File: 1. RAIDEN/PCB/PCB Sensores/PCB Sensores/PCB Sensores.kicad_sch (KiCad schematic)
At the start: 19 parts, among them J2 LEDS_1, J3 LEDS_1, J4 LEDS_1, U1 BOB-09056

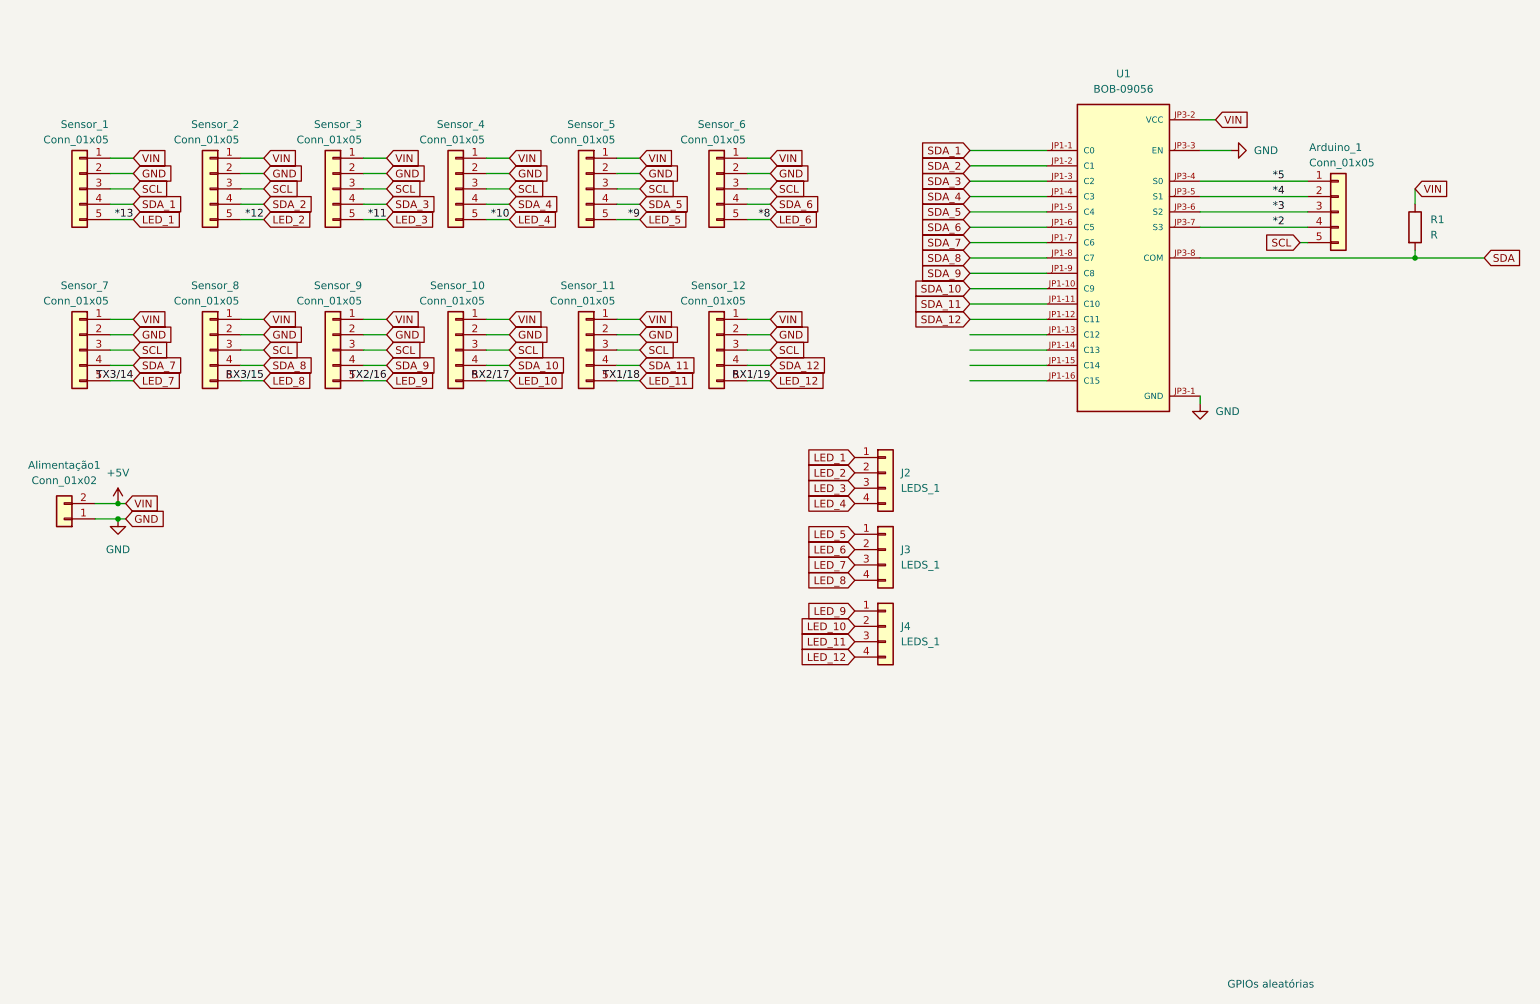
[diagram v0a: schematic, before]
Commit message: V2 da PCB dos sensores
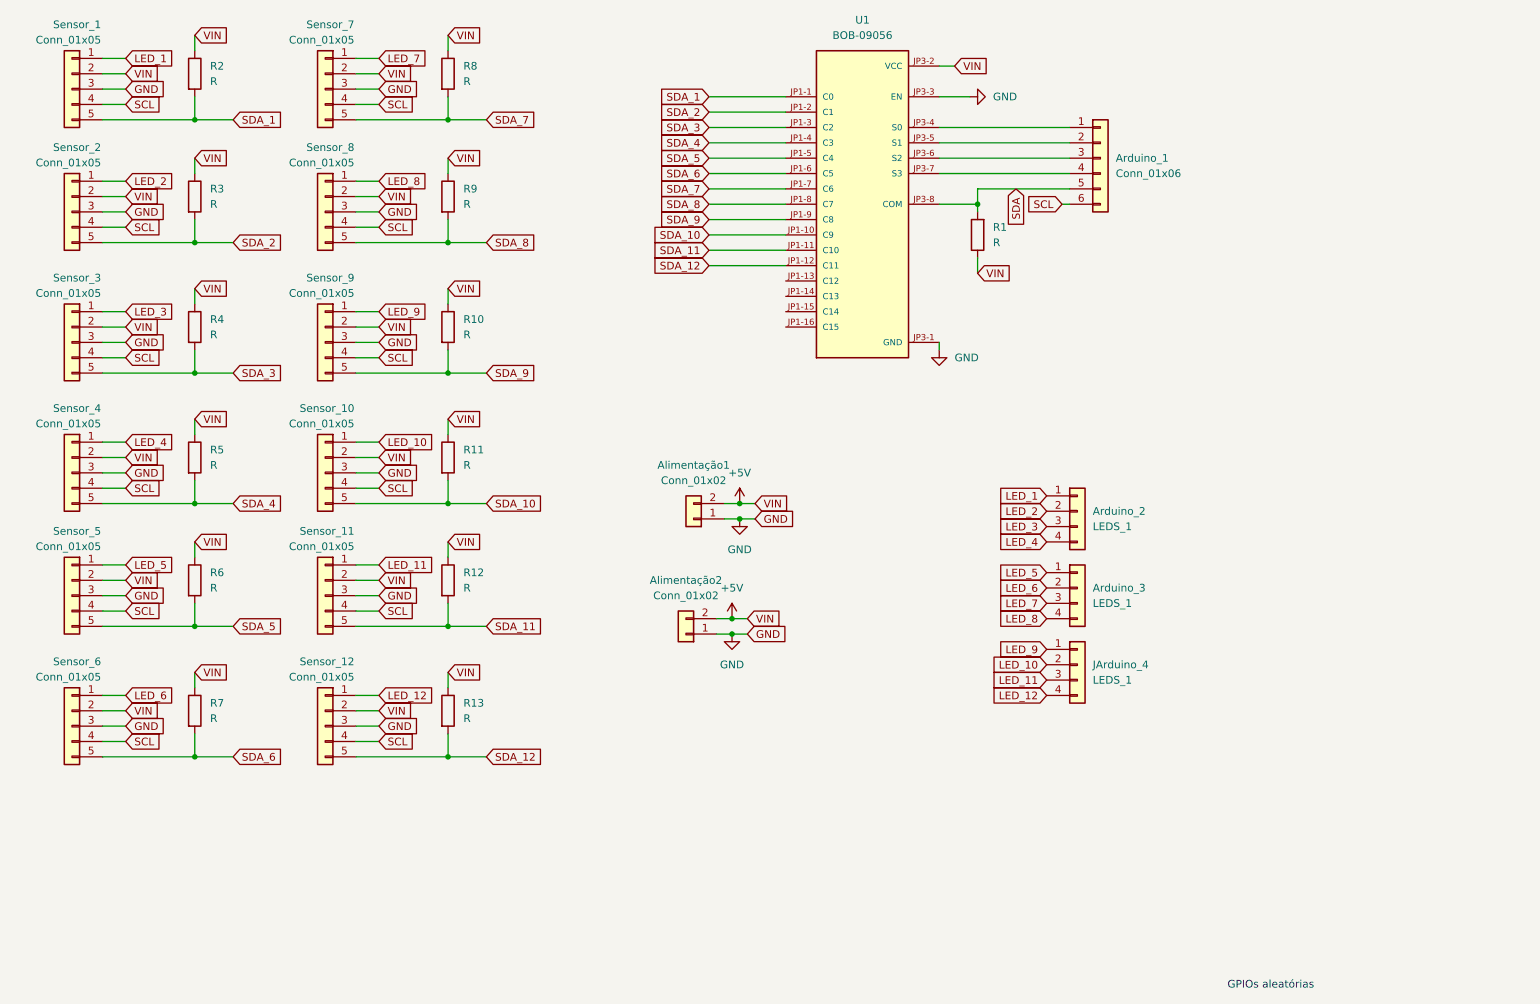
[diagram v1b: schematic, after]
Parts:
- removed Arduino_1: Conn_01x05, Connector_PinSocket_2.54mm:PinSocket_1x05_P2.54mm_Vertical, symbol Connector_Generic:Conn_01x05
- added Alimentação2: Conn_01x02, Connector_PinSocket_2.54mm:PinSocket_1x02_P2.54mm_Vertical, symbol Connector_Generic:Conn_01x02
- added Arduino_1: Conn_01x06, Connector_PinHeader_2.54mm:PinHeader_1x06_P2.54mm_Vertical, symbol Connector_Generic:Conn_01x06
- added R10, R11, R12, R13, R2, R3, R4, R5, R6, R7, R8, R9: R, Resistor_THT:R_Axial_DIN0207_L6.3mm_D2.5mm_P7.62mm_Horizontal, symbol Device:R
- renumbered J2 to Arduino_2, J3 to Arduino_3, J4 to JArduino_4
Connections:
- net +5V: now also Sensor_1.2 (Pin_2), Sensor_10.2 (Pin_2), Sensor_11.2 (Pin_2), Sensor_12.2 (Pin_2), Sensor_2.2 (Pin_2), Sensor_3.2 (Pin_2), Sensor_4.2 (Pin_2), Sensor_5.2 (Pin_2), Sensor_6.2 (Pin_2), Sensor_7.2 (Pin_2), Sensor_8.2 (Pin_2), Sensor_9.2 (Pin_2), Alimentação2.2 (Pin_2), R10.1, R11.1, R12.1, R13.1, R2.1, R3.1, R4.1, R5.1, R6.1, R7.1, R8.1, R9.1; no longer Sensor_1.1 (Pin_1), Sensor_10.1 (Pin_1), Sensor_11.1 (Pin_1), Sensor_12.1 (Pin_1), Sensor_2.1 (Pin_1), Sensor_3.1 (Pin_1), Sensor_4.1 (Pin_1), Sensor_5.1 (Pin_1), Sensor_6.1 (Pin_1), Sensor_7.1 (Pin_1), Sensor_8.1 (Pin_1), Sensor_9.1 (Pin_1)
- net GND: now also Sensor_1.3 (Pin_3), Sensor_10.3 (Pin_3), Sensor_11.3 (Pin_3), Sensor_12.3 (Pin_3), Sensor_2.3 (Pin_3), Sensor_3.3 (Pin_3), Sensor_4.3 (Pin_3), Sensor_5.3 (Pin_3), Sensor_6.3 (Pin_3), Sensor_7.3 (Pin_3), Sensor_8.3 (Pin_3), Sensor_9.3 (Pin_3), Alimentação2.1 (Pin_1); no longer Sensor_1.2 (Pin_2), Sensor_10.2 (Pin_2), Sensor_11.2 (Pin_2), Sensor_12.2 (Pin_2), Sensor_2.2 (Pin_2), Sensor_3.2 (Pin_2), Sensor_4.2 (Pin_2), Sensor_5.2 (Pin_2), Sensor_6.2 (Pin_2), Sensor_7.2 (Pin_2), Sensor_8.2 (Pin_2), Sensor_9.2 (Pin_2)
- net LED_1: now also Sensor_1.1 (Pin_1); no longer Sensor_1.5 (Pin_5)
- net LED_10: now also Sensor_10.1 (Pin_1); no longer Sensor_10.5 (Pin_5)
- net LED_11: now also Sensor_11.1 (Pin_1); no longer Sensor_11.5 (Pin_5)
- net LED_12: now also Sensor_12.1 (Pin_1); no longer Sensor_12.5 (Pin_5)
- net LED_2: now also Sensor_2.1 (Pin_1); no longer Sensor_2.5 (Pin_5)
- net LED_3: now also Sensor_3.1 (Pin_1); no longer Sensor_3.5 (Pin_5)
- net LED_4: now also Sensor_4.1 (Pin_1); no longer Sensor_4.5 (Pin_5)
- net LED_5: now also Sensor_5.1 (Pin_1); no longer Sensor_5.5 (Pin_5)
- net LED_6: now also Sensor_6.1 (Pin_1); no longer Sensor_6.5 (Pin_5)
- net LED_7: now also Sensor_7.1 (Pin_1); no longer Sensor_7.5 (Pin_5)
- net LED_8: now also Sensor_8.1 (Pin_1); no longer Sensor_8.5 (Pin_5)
- net LED_9: now also Sensor_9.1 (Pin_1); no longer Sensor_9.5 (Pin_5)
- net SCL: now also Sensor_1.4 (Pin_4), Sensor_10.4 (Pin_4), Sensor_11.4 (Pin_4), Sensor_12.4 (Pin_4), Sensor_2.4 (Pin_4), Sensor_3.4 (Pin_4), Sensor_4.4 (Pin_4), Sensor_5.4 (Pin_4), Sensor_6.4 (Pin_4), Sensor_7.4 (Pin_4), Sensor_8.4 (Pin_4), Sensor_9.4 (Pin_4), Arduino_1.6 (Pin_6); no longer Sensor_1.3 (Pin_3), Sensor_10.3 (Pin_3), Sensor_11.3 (Pin_3), Sensor_12.3 (Pin_3), Sensor_2.3 (Pin_3), Sensor_3.3 (Pin_3), Sensor_4.3 (Pin_3), Sensor_5.3 (Pin_3), Sensor_6.3 (Pin_3), Sensor_7.3 (Pin_3), Sensor_8.3 (Pin_3), Sensor_9.3 (Pin_3)
- net SDA: now also Arduino_1.5 (Pin_5)
- net SDA_1: now also Sensor_1.5 (Pin_5), R2.2; no longer Sensor_1.4 (Pin_4)
- net SDA_10: now also Sensor_10.5 (Pin_5), R11.2; no longer Sensor_10.4 (Pin_4)
- net SDA_11: now also Sensor_11.5 (Pin_5), R12.2; no longer Sensor_11.4 (Pin_4)
- net SDA_12: now also Sensor_12.5 (Pin_5), R13.2; no longer Sensor_12.4 (Pin_4)
- net SDA_2: now also Sensor_2.5 (Pin_5), R3.2; no longer Sensor_2.4 (Pin_4)
- net SDA_3: now also Sensor_3.5 (Pin_5), R4.2; no longer Sensor_3.4 (Pin_4)
- net SDA_4: now also Sensor_4.5 (Pin_5), R5.2; no longer Sensor_4.4 (Pin_4)
- net SDA_5: now also Sensor_5.5 (Pin_5), R6.2; no longer Sensor_5.4 (Pin_4)
- net SDA_6: now also Sensor_6.5 (Pin_5), R7.2; no longer Sensor_6.4 (Pin_4)
- net SDA_7: now also Sensor_7.5 (Pin_5), R8.2; no longer Sensor_7.4 (Pin_4)
- net SDA_8: now also Sensor_8.5 (Pin_5), R9.2; no longer Sensor_8.4 (Pin_4)
- net SDA_9: now also Sensor_9.5 (Pin_5), R10.2; no longer Sensor_9.4 (Pin_4)
- net *2: no longer names the net of U1.JP3-7 (S3)
- net *2: now also Arduino_1.4 (Pin_4)
- net *3: no longer names the net of U1.JP3-6 (S2)
- net *3: now also Arduino_1.3 (Pin_3)
- net *4: no longer names the net of U1.JP3-5 (S1)
- net *4: now also Arduino_1.2 (Pin_2)
- net *5: no longer names the net of U1.JP3-4 (S0)
- net *5: now also Arduino_1.1 (Pin_1)
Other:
- moved on the sheet: Alimentação1, Arduino_2, Arduino_3, JArduino_4, R1, Sensor_1, Sensor_10, Sensor_11, Sensor_12, Sensor_2, Sensor_3, Sensor_4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
